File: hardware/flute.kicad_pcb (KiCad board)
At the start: 2 copper layers, 230 x 20 mm, 47 parts, among them J1 Conn_01x02, J3 Conn_01x04, SW1 C, SW2 D, SW3 E, SW4 F, SW5 G, SW6 A, SW7 H, SW8 OCTAVE?, U1 RP2040, U2 W25Q128JVS, Y1 Crystal_GND24

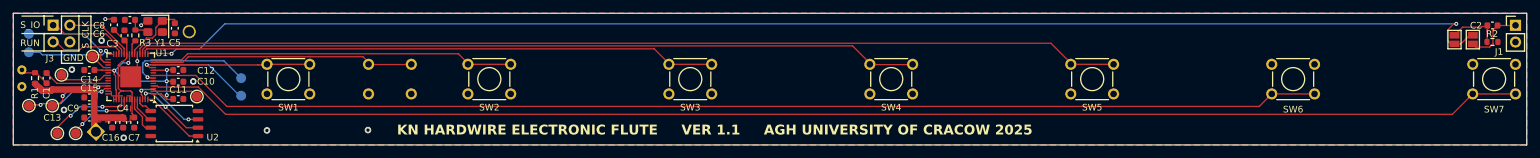
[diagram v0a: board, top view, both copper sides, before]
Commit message: complete pcb ver1.1
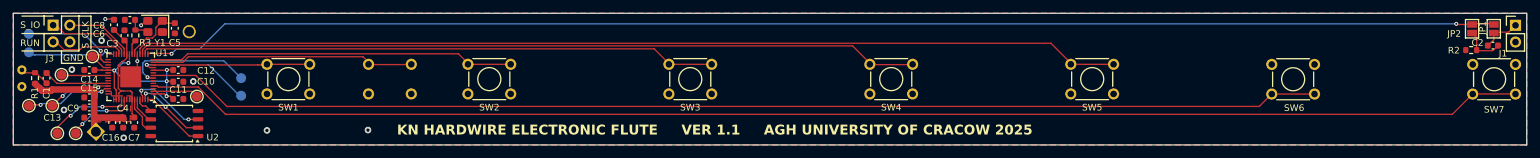
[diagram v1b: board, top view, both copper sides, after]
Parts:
- moved JP2 3.58 mm to (258.7, 103.7)
- moved R2 3.46 mm to (255.3, 107.0), turned to 180 degrees
- moved JP1 3.14 mm to (255.4, 103.7), turned to 90 degrees
- moved C2 3.05 mm to (258.6, 106.3), turned to 0 degrees
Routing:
- net Net-(J1-Pin_1): track 9.25 -> 6.14 mm
- net /PWM_OUT: track 208.7 -> 206.6 mm
- net Net-(JP1-A): track 8.17 -> 6.49 mm
